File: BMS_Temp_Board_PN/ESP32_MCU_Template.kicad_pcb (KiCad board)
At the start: 4 copper layers, 185.6 x 74 mm, 66 parts, among them IC1 ESP32-S3-WROOM-1-N8R8, IC10 CD74HC4067PWR, IC11 CD74HC4067PWR, IC12 CD74HC4067PWR, IC13 CD74HC4067PWR, IC14 CD74HC4067PWR, IC15 CD74HC4067PWR, IC2 CP2102N-A02-GQFN28, IC3 TLP175A_TPL,E, IC4 TPS2116DRLR, IC5 MIC37100-3.3WS, IC6 CD74HC4067PWR, IC7 CD74HC4067PWR, IC8 CD74HC4067PWR, IC9 CD74HC4067PWR, J1 ESP_USB, J10 B32B-PUDSS-1_LF__SN_, J11 B32B-PUDSS-1_LF__SN_, J12 B2B-PH-K-S, J2 B32B-PUDSS-1_LF__SN_, J3 B32B-PUDSS-1_LF__SN_, J4 B32B-PUDSS-1_LF__SN_, J5 B32B-PUDSS-1_LF__SN_, J6 B32B-PUDSS-1_LF__SN_, J7 B32B-PUDSS-1_LF__SN_, J8 B32B-PUDSS-1_LF__SN_, J9 B32B-PUDSS-1_LF__SN_, Q1 MMBT2222LT1G, Q2 MMBT2222LT1G, U1 USBLC6-2SC6, U2 SN65HVD230

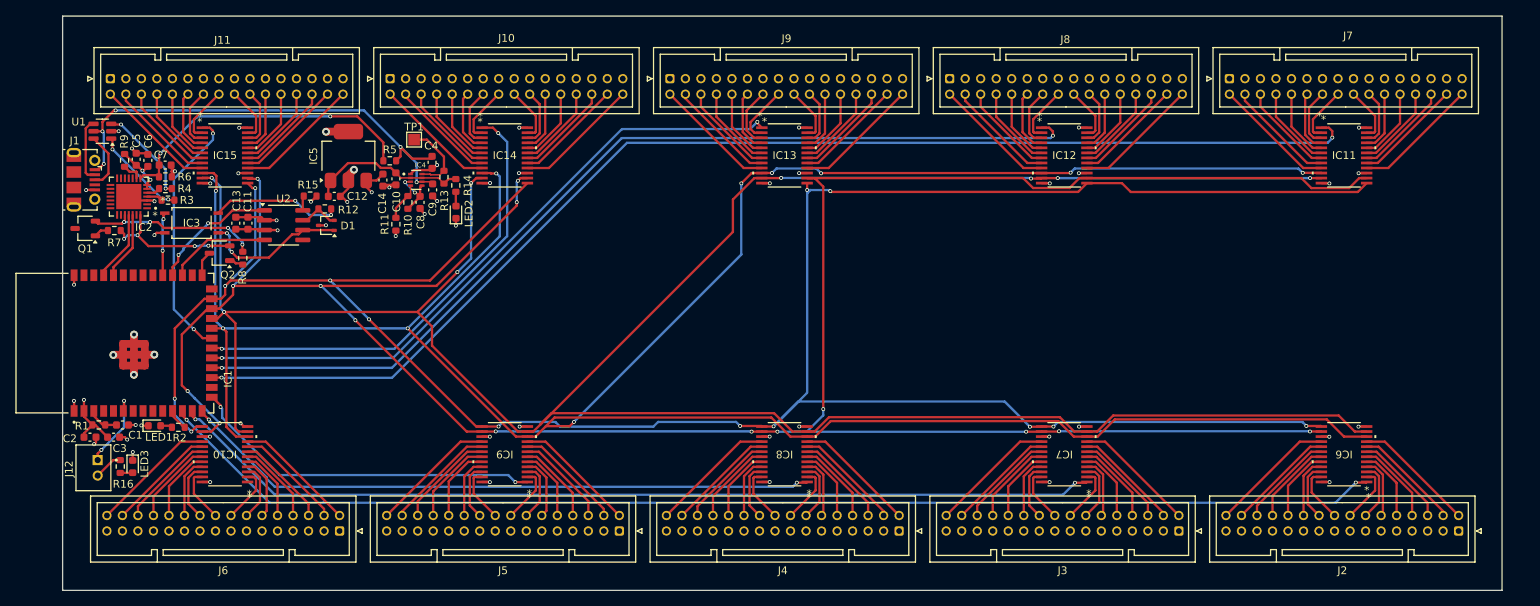
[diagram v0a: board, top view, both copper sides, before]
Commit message: (hopefully) final revision of the bms temp board
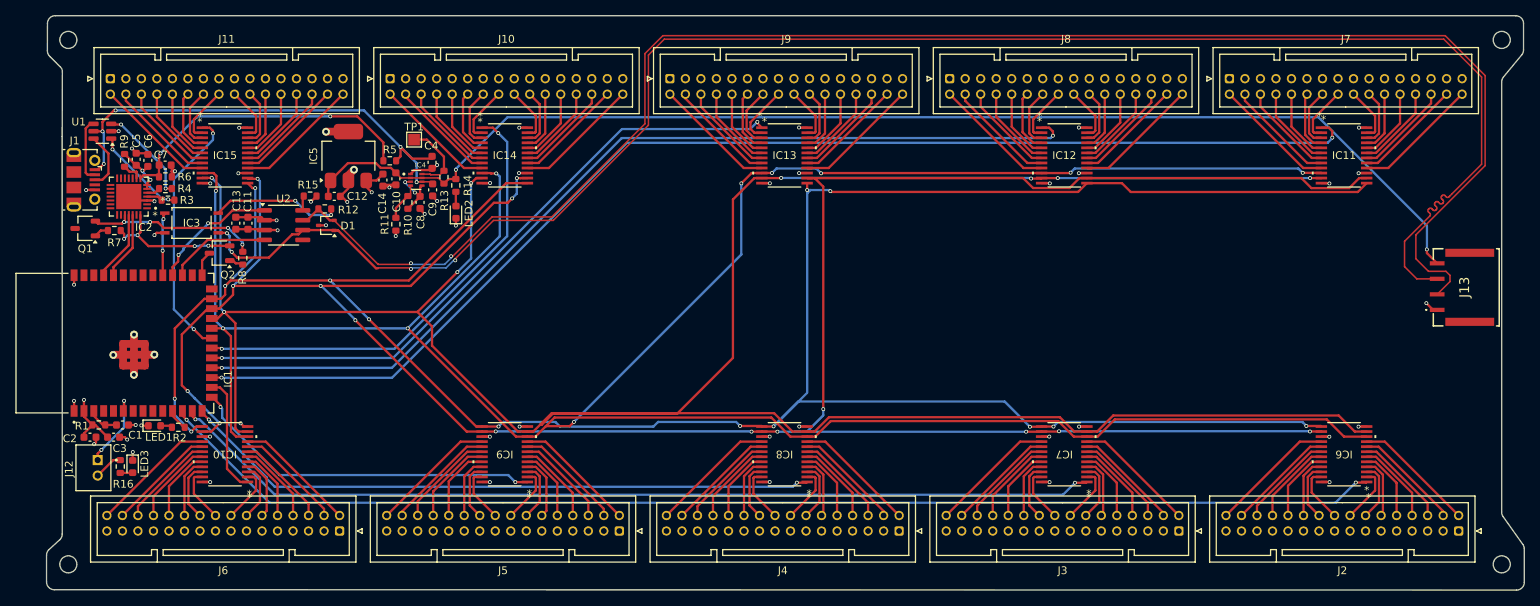
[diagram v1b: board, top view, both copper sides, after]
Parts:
- added H1: MountingHole, MountingHole:MountingHole_2.2mm_M2, F.Cu at (235.4, 65.8)
- added H2: MountingHole, MountingHole:MountingHole_2.2mm_M2, F.Cu at (235.4, 133.4)
- added H3: MountingHole, MountingHole:MountingHole_2.2mm_M2, F.Cu at (50.5, 133.4)
- added H4: MountingHole, MountingHole:MountingHole_2.2mm_M2, F.Cu at (50.5, 65.8)
- added J13: SM04B-ULHK-1TA1-ETB_HF_, SM04B-ULH:SM04BULHK1TA1ETBHF, F.Cu at (230.8, 97.7)
- J10, J11, J2, J3, J4, J5, J6, J7, J8, J9: footprint Connector_JST:JST_PUD_B32B-PUDSS_2x16_P2.00mm_Vertical -> ESP32_S3_WROOM_1_N8R8:JST_PUD_B32B-PUDSS_2x16_P2.00mm_Vertical_PN
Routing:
- net /CAN+: track 5.26 -> 211.6 mm, vias 0 -> 2
- net /CAN-: track 18.8 -> 225.1 mm, vias 2 -> 4
- net +5V: track 20.6 -> 161.1 mm, vias 0 -> 2
- net /MUX5: track 0.00 -> 15.3 mm
- net /MUX_S1: track 336.4 -> 345.9 mm
- net GND: track 89.5 -> 91.2 mm, vias 49 -> 50
- net /MUX_S2: track 334.4 -> 333.8 mm
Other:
- board size 185.6 x 74 mm -> 190.5 x 74.1 mm
